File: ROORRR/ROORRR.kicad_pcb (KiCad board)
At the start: 2 copper layers, 205.6 x 87.3 mm, 92 parts, among them J1 AVR-ISP-6, SW1 SW_Push, U1 ATmega32U4-AU, U2 PRTR5V0U2X, Y1 16MHz

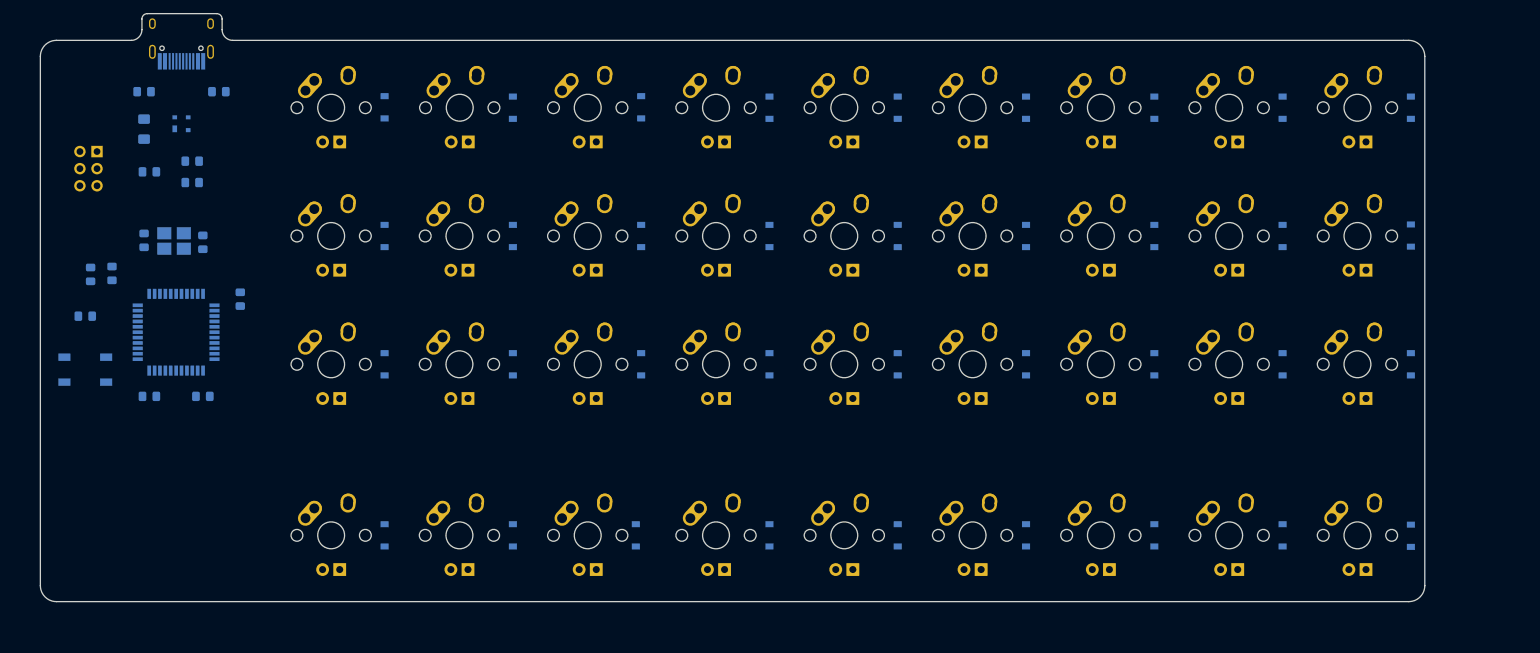
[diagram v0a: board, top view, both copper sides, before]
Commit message: checkpoint 2
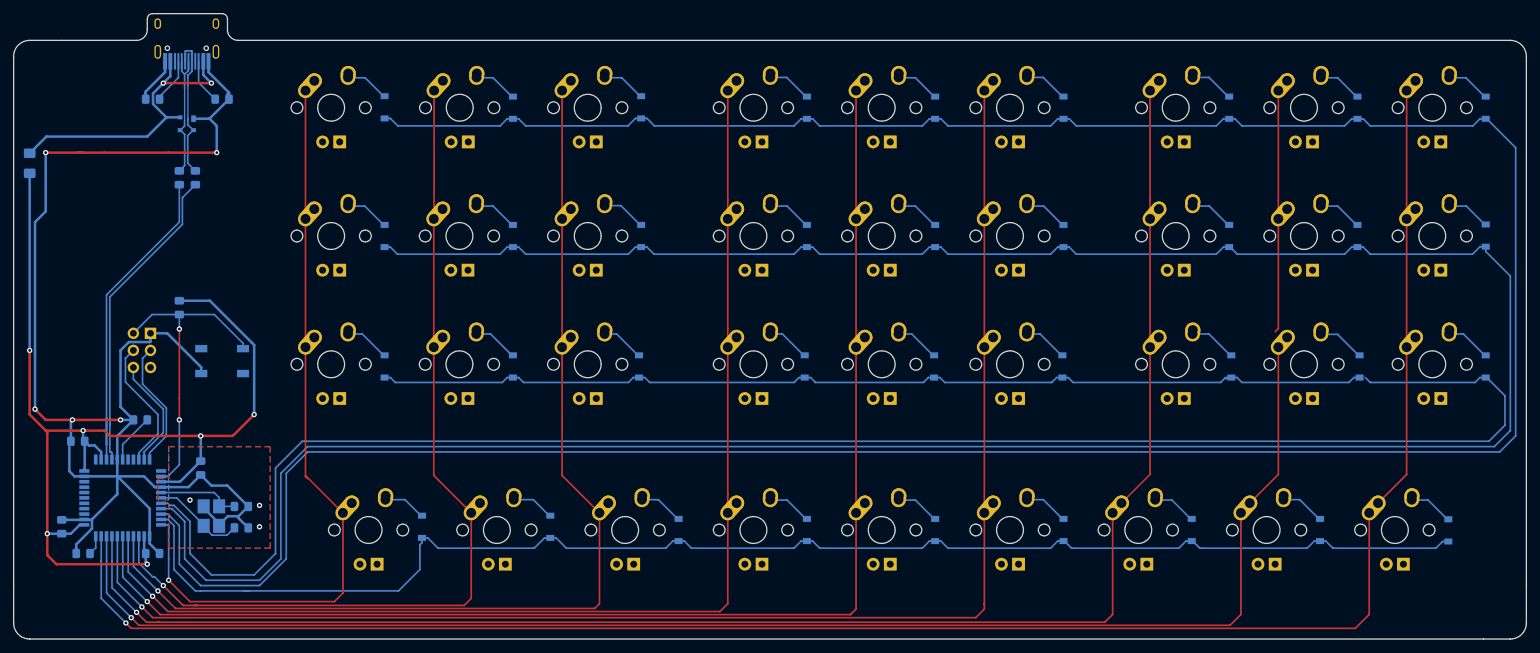
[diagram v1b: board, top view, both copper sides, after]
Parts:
- removed C4: 0.1uF, Capacitor_SMD:C_0805_2012Metric_Pad1.15x1.40mm_HandSolder
- added C8: 0.1uF, Capacitor_SMD:C_0805_2012Metric_Pad1.15x1.40mm_HandSolder, B.Cu at (73.0, 115.9)
- moved R4 57.5 mm to (62.7, 115.9)
- moved C1 42.8 mm to (86.2, 112.1), turned to 0 degrees
- moved C2 42.1 mm to (86.2, 108.9), turned to 0 degrees
- moved Y1 41.2 mm to (81.8, 110.3), turned to 90 degrees
- moved C6 28.5 mm to (59.5, 111.9), turned to 90 degrees
- moved J1 28.1 mm to (71.4, 85.7)
- moved U1 25.9 mm to (68.6, 107.6), turned to 270 degrees
- moved C5 25.7 mm to (80.2, 103.2), turned to 270 degrees
- moved SW1 20.4 mm to (83.3, 87.3)
- moved F1 17.7 mm to (54.8, 57.9), turned to 270 degrees
- moved C3 17.4 mm to (71.2, 96.0), turned to 180 degrees
- moved R1 14.1 mm to (77.0, 79.4), turned to 270 degrees
- moved C7 12.6 mm to (61.9, 99.2)
- moved D27 11.4 mm to (233.2, 88.1), turned to 90 degrees
- moved D28 11.4 mm to (252.3, 88.1), turned to 90 degrees
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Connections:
- net Net-(C1-Pad1) renamed XTAL1
- net Net-(C2-Pad1) renamed XTAL2
- D1 pad 1: Col0 -> Row0
- D11 pad 1: Col0 -> Row1
- D12 pad 1: Col0 -> Row1
- D13 pad 1: Col0 -> Row1
- D14 pad 1: Col0 -> Row1
- D15 pad 1: Col0 -> Row1
- D16 pad 1: Col0 -> Row1
- D17 pad 1: Col0 -> Row1
- D18 pad 1: Col0 -> Row1
- D19 pad 1: Col0 -> Row1
- D2 pad 1: Col0 -> Row0
- D21 pad 1: Col0 -> Row2
- D22 pad 1: Col0 -> Row2
- D23 pad 1: Col0 -> Row2
- D24 pad 1: Col0 -> Row2
- D25 pad 1: Col0 -> Row2
- D26 pad 1: Col0 -> Row2
- D27 pad 1: Col0 -> Row2
- D28 pad 1: Col0 -> Row2
- D29 pad 1: Col0 -> Row2
- D3 pad 1: Col0 -> Row0
- D31 pad 1: Col0 -> Row3
- D32 pad 1: Col0 -> Row3
- D33 pad 1: Col0 -> Row3
- D34 pad 1: Col0 -> Row3
- D35 pad 1: Col0 -> Row3
- D36 pad 1: Col0 -> Row3
- D37 pad 1: Col0 -> Row3
- D38 pad 1: Col0 -> Row3
- D39 pad 1: Col0 -> Row3
- D4 pad 1: Col0 -> Row0
- D5 pad 1: Col0 -> Row0
- D6 pad 1: Col0 -> Row0
- D7 pad 1: Col0 -> Row0
- D8 pad 1: Col0 -> Row0
- D9 pad 1: Col0 -> Row0
- MX12 pad 1: Col0 -> Col1
- MX13 pad 1: Col0 -> Col2
- MX14 pad 1: Col0 -> Col3
- MX15 pad 1: Col0 -> Col4
- MX16 pad 1: Col0 -> Col5
- MX17 pad 1: Col0 -> Col6
- MX18 pad 1: Col0 -> Col7
- MX19 pad 1: Col0 -> Col8
- MX2 pad 1: Col0 -> Col1
- MX22 pad 1: Col0 -> Col1
- MX23 pad 1: Col0 -> Col2
- MX24 pad 1: Col0 -> Col3
- MX25 pad 1: Col0 -> Col4
- MX26 pad 1: Col0 -> Col5
- MX27 pad 1: Col0 -> Col6
- MX28 pad 1: Col0 -> Col7
- MX29 pad 1: Col0 -> Col8
- MX3 pad 1: Col0 -> Col2
- MX32 pad 1: Col0 -> Col1
- MX33 pad 1: Col0 -> Col2
- MX34 pad 1: Col0 -> Col3
- MX35 pad 1: Col0 -> Col4
- MX36 pad 1: Col0 -> Col5
- MX37 pad 1: Col0 -> Col6
- MX38 pad 1: Col0 -> Col7
- MX39 pad 1: Col0 -> Col8
- MX4 pad 1: Col0 -> Col3
- MX5 pad 1: Col0 -> Col4
- MX6 pad 1: Col0 -> Col5
- MX7 pad 1: Col0 -> Col6
- MX8 pad 1: Col0 -> Col7
- MX9 pad 1: Col0 -> Col8
- R1 pad 2: Net-(R1-Pad2) -> RESET
- SW1 pad 2: Net-(R1-Pad2) -> RESET
- U1 pad 10: MOSI -> MISO
- U1 pad 11: MISO -> MOSI
- U1 pad 13: Net-(R1-Pad2) -> RESET
- U1 pad 18: Net-(U1-Pad18) -> Row2
- U1 pad 19: Net-(U1-Pad19) -> Row1
- U1 pad 20: Net-(U1-Pad20) -> Row0
- U1 pad 21: Net-(U1-Pad21) -> Row3
- U1 pad 22: Net-(U1-Pad22) -> Col0
- U1 pad 25: Net-(U1-Pad25) -> Col1
- U1 pad 26: Net-(U1-Pad26) -> Col2
- U1 pad 27: Net-(U1-Pad27) -> Col3
- U1 pad 28: Net-(U1-Pad28) -> Col4
- U1 pad 29: Net-(U1-Pad29) -> Col5
- U1 pad 30: Net-(U1-Pad30) -> Col6
- U1 pad 31: Net-(U1-Pad31) -> Col7
- U1 pad 32: Net-(U1-Pad32) -> Col8
- USB1 pad 1: Net-(USB1-Pad1) -> GND
- USB1 pad 13: Net-(USB1-Pad1) -> GND
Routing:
- net Row0: track 0.00 -> 445.3 mm
- net Row1: track 0.00 -> 424.0 mm
- net Row2: track 0.00 -> 400.1 mm
- net Col8: track 0.00 -> 278.3 mm, vias 0 -> 1
- net Col7: track 0.00 -> 257.5 mm, vias 0 -> 1
- net Col6: track 0.00 -> 237.1 mm, vias 0 -> 1
- net GND: track 0.00 -> 225.8 mm, vias 0 -> 8
- net Col5: track 0.00 -> 215.4 mm, vias 0 -> 1
- net Row3: track 0.00 -> 213.5 mm
- net Col4: track 0.00 -> 195.4 mm, vias 0 -> 1
- net Col3: track 0.00 -> 173.4 mm, vias 0 -> 1
- net +5V: track 0.00 -> 161.8 mm, vias 0 -> 6
- net Col2: track 0.00 -> 155.1 mm, vias 0 -> 1
- net Col1: track 0.00 -> 134.5 mm, vias 0 -> 1
- net Col0: track 0.00 -> 115.3 mm, vias 0 -> 1
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- added copper zone on F.Cu, net (none)
- added copper zone on B.Cu, net GND
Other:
- board size 205.6 x 87.3 mm -> 224.6 x 92.9 mm
